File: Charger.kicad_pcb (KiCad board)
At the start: 2 copper layers, 71.8 x 43.8 mm, 43 parts, among them J1 Input, J2 USB-A-S-X-X-SM2, J3 USB-A-S-X-X-SM2, Q1 BSC42DN25NS3, T1 760875131, U1 LT1085-5.0, U2 TPS2546, U3 LT3798MPMSETRPBF, U4 TPS2546RTER

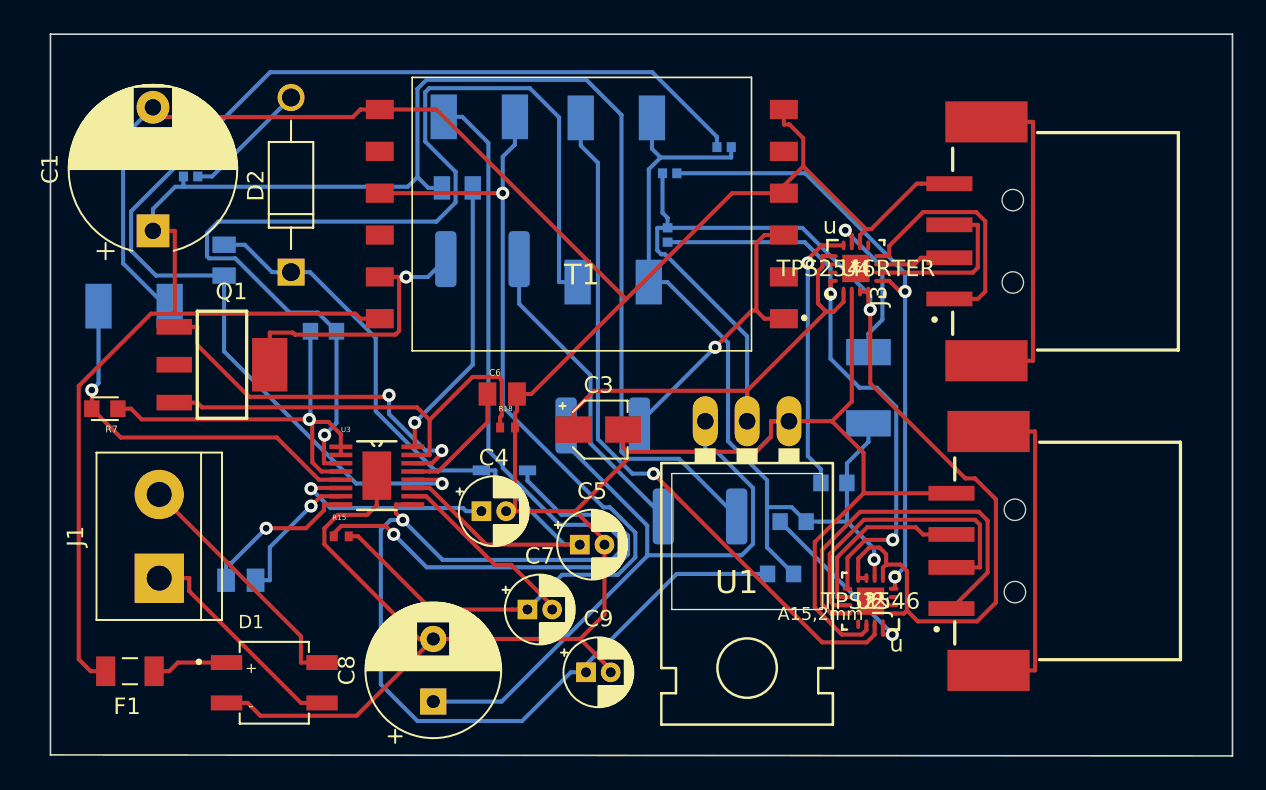
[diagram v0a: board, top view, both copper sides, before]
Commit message: compact
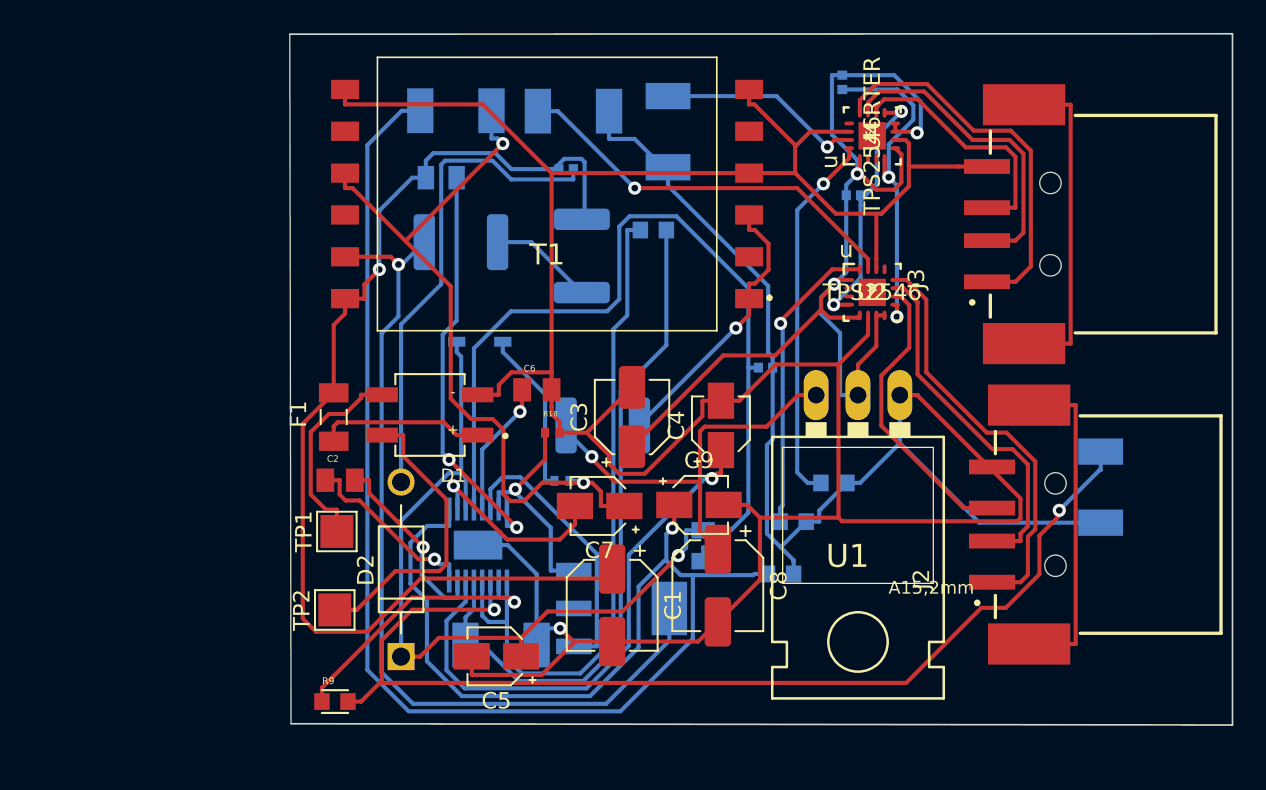
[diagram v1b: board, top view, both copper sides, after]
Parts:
- removed J1: Input, TerminalBlock:TerminalBlock_bornier-2_P5.08mm
- added TP1: TestPoint, TestPoint:TestPoint_Pad_2.0x2.0mm, F.Cu at (79.0, 59.4)
- added TP2: TestPoint, TestPoint:TestPoint_Pad_2.0x2.0mm, F.Cu at (78.9, 64.2)
- C1: footprint Capacitor_THT:CP_Radial_D10.0mm_P7.50mm -> Capacitor_SMD:CP_Elec_5x4.4
- C2, R9: moved to F.Cu
- C3: footprint Capacitor_SMD:CP_Elec_3x5.3 -> Capacitor_SMD:CP_Elec_4x3.9
- C4, C5, C7, C9: footprint Capacitor_THT:CP_Radial_D4.0mm_P1.50mm -> Capacitor_SMD:CP_Elec_3x5.3
- C8: footprint Capacitor_THT:CP_Radial_D8.0mm_P3.80mm -> Capacitor_SMD:CP_Elec_5x4.4
- Q1, R15, R7, U3: moved to B.Cu
- moved C1 36.0 mm to (95.7, 63.9), turned to 270 degrees
- moved R7 35.0 mm to (98.2, 41.1), turned to 0 degrees
- moved R13 33.9 mm to (101.2, 60.3)
- moved R10 32.1 mm to (125.3, 56.7), turned to 270 degrees
- moved R8 30.3 mm to (89.0, 66.3)
- moved Q1 28.4 mm to (96.3, 64.1)
- moved D2 24.3 mm to (82.9, 61.7)
- moved R12 22.8 mm to (92.9, 37.4)
- moved R9 22.5 mm to (78.9, 69.7)
- moved F1 19.8 mm to (78.8, 52.5), turned to 90 degrees
- moved R5 19.7 mm to (99.1, 35.1)
- moved D1 18.8 mm to (84.6, 52.3), turned to 180 degrees
- moved U2 18.7 mm to (111.5, 44.9), turned to 0 degrees
- moved C8 18.7 mm to (102.1, 62.7), turned to 270 degrees
- moved D4 17.4 mm to (93.9, 42.7), turned to 90 degrees
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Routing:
- net Net-(C1-Pad1): track 113.6 -> 67.2 mm, vias 0 -> 1
- net Net-(D5-Pad1): track 17.7 -> 52.5 mm
- net Vint: track 99.2 -> 65.0 mm, vias 1 -> 3
- net Net-(R7-Pad1): track 25.2 -> 59.0 mm
- net Stat2: track 37.7 -> 15.7 mm
- net Net-(D2-PadA): track 7.65 -> 29.5 mm
- net Net-(C4-Pad1): track 12.7 -> 33.1 mm
- net en: track 73.0 -> 52.8 mm, vias 1 -> 0
- net Net-(D3-PadA): track 28.8 -> 10.1 mm, vias 1 -> 0
- net Net-(R7-Pad2): track 23.3 -> 41.7 mm, vias 1 -> 0
- net Net-(R3-Pad1): track 42.7 -> 24.4 mm
- net Net-(C8-Pad1): track 42.4 -> 25.4 mm, vias 0 -> 1
- net Net-(C9-Pad1): track 89.2 -> 104.9 mm
- net Stat1: track 35.3 -> 20.4 mm
- net DM2: track 4.44 -> 19.1 mm
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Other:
- board size 71.8 x 43.8 mm -> 57.2 x 42 mm

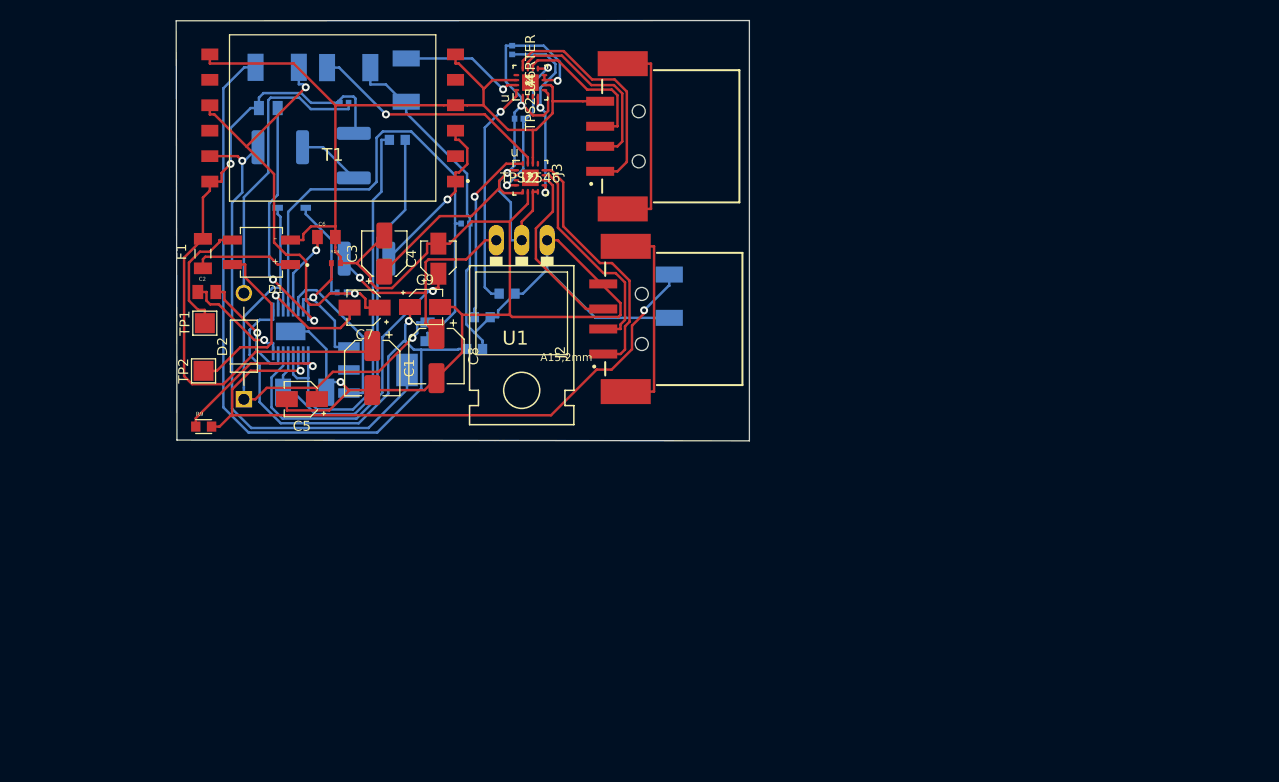
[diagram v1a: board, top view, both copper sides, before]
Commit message: updates
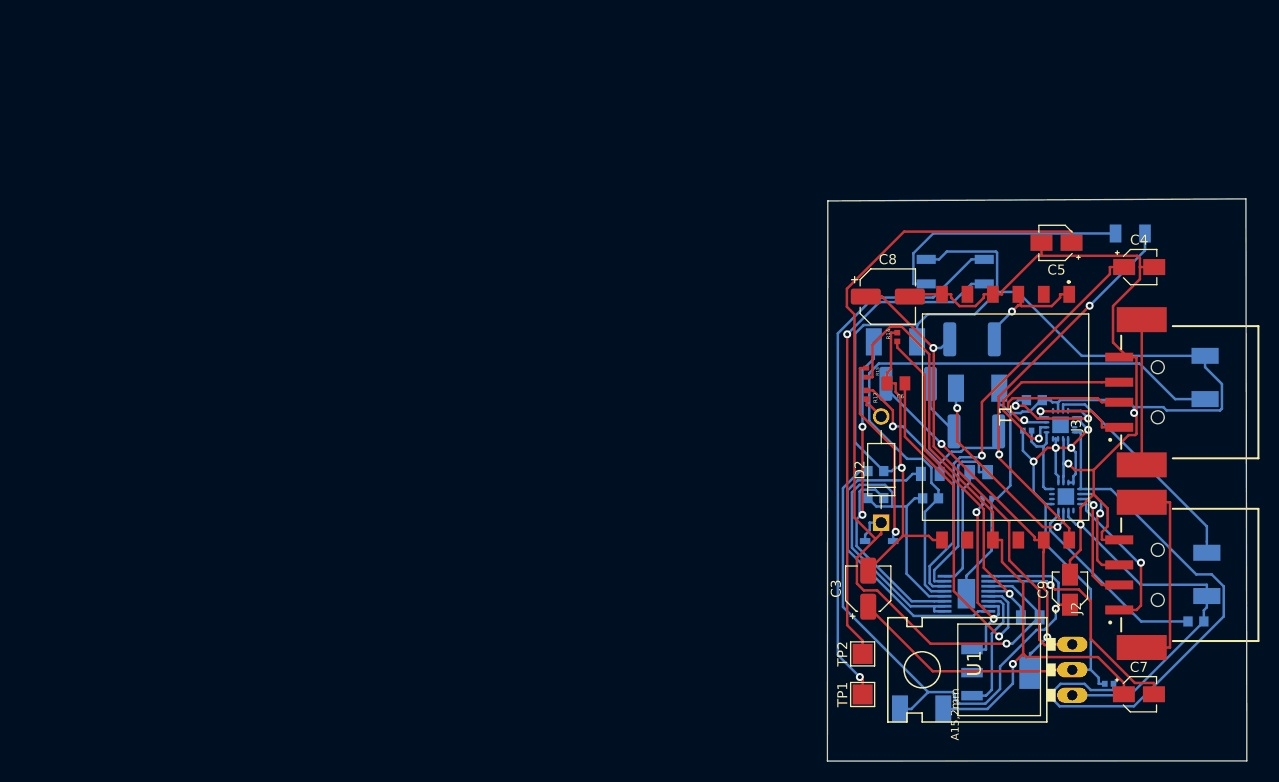
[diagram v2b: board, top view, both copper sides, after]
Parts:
- removed C1: 470u, Capacitor_SMD:CP_Elec_5x4.4
- C2, D1, F1, R18, R9, U2, U4: moved to B.Cu
- R12, R14, R15: moved to F.Cu
- moved R5 93.9 mm to (179.0, 84.5)
- moved F1 92.6 mm to (171.4, 50.4), turned to 0 degrees
- moved R16 90.8 mm to (150.5, 97.9)
- moved R8 89.9 mm to (178.8, 64.8), turned to 90 degrees
- moved R1 86.9 mm to (169.3, 95.4), turned to 0 degrees
- moved C7 86.4 mm to (172.2, 96.4), turned to 0 degrees
- moved C2 79.1 mm to (156.2, 74.3)
- moved R4 77.5 mm to (177.9, 89.2)
- moved C5 76.9 mm to (164.0, 51.4)
- moved R11 75.5 mm to (151.4, 74.4), turned to 180 degrees
- moved TP1 75.4 mm to (144.7, 96.5)
- moved T1 73.5 mm to (158.9, 68.8), turned to 270 degrees
- moved U3 72.4 mm to (155.0, 86.4), turned to 0 degrees
- moved TP2 71.6 mm to (144.7, 92.4)
- moved R3 70.5 mm to (156.1, 65.9)
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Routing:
- net VinL: track 46.7 -> 90.8 mm
- net Net-(C9-Pad1): track 104.9 -> 61.6 mm
- net AC1: track 12.5 -> 54.8 mm, vias 0 -> 1
- net Stat1: track 20.4 -> 56.8 mm, vias 2 -> 0
- net AC2: track 18.1 -> 48.3 mm, vias 0 -> 1
- net Net-(R10-Pad1): track 66.2 -> 37.5 mm
- net Net-(D2-PadA): track 29.5 -> 2.52 mm
- net Net-(C6-Pad1): track 8.24 -> 35.2 mm
- net gnd: track 247.5 -> 272.9 mm, vias 1 -> 4
- net dcm: track 45.3 -> 69.5 mm, vias 2 -> 1
- net Net-(C8-Pad1): track 25.4 -> 47.9 mm
- net Net-(R7-Pad2): track 41.7 -> 63.1 mm
- net en: track 52.8 -> 34.9 mm, vias 0 -> 1
- net Net-(R7-Pad1): track 59.0 -> 42.4 mm, vias 1 -> 0
- net Net-(D5-Pad1): track 52.5 -> 36.9 mm, vias 1 -> 2
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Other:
- board size 57.2 x 42 mm -> 41.9 x 56.1 mm
